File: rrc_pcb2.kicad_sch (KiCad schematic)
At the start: 15 parts, among them J1 buzzer_toggle_pin, J2 battery_header, U1 BN220-GPS, U2 INA260, U3 Teensy4.1, U4 voltReg, U5 MS5611, U6 logo

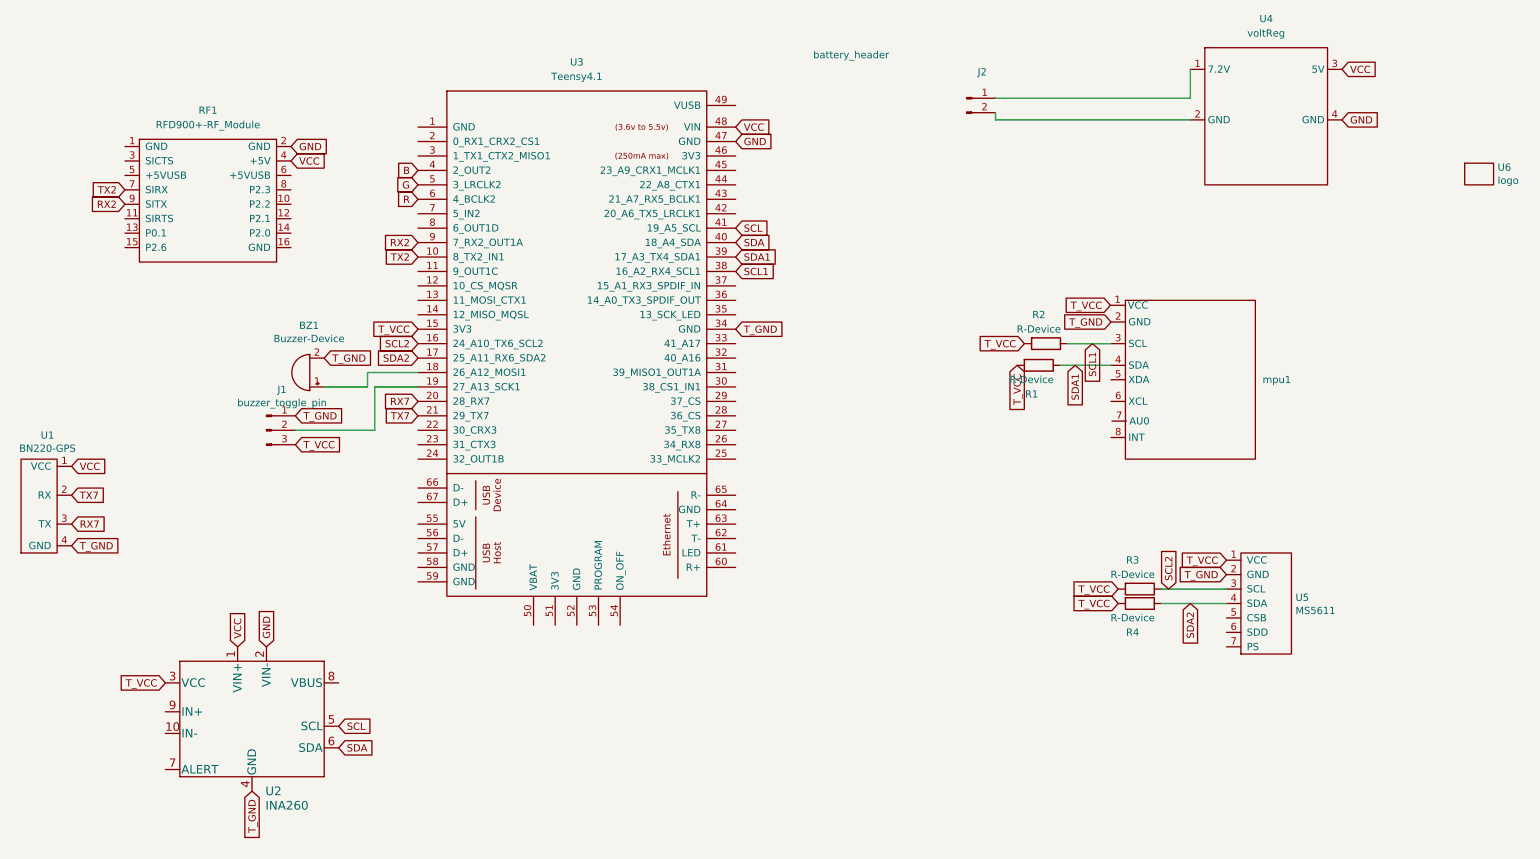
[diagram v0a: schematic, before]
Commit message: big cleanup of files
also new teensy4.1 symbo(the accurate one now) and fixed rfd900 schematic
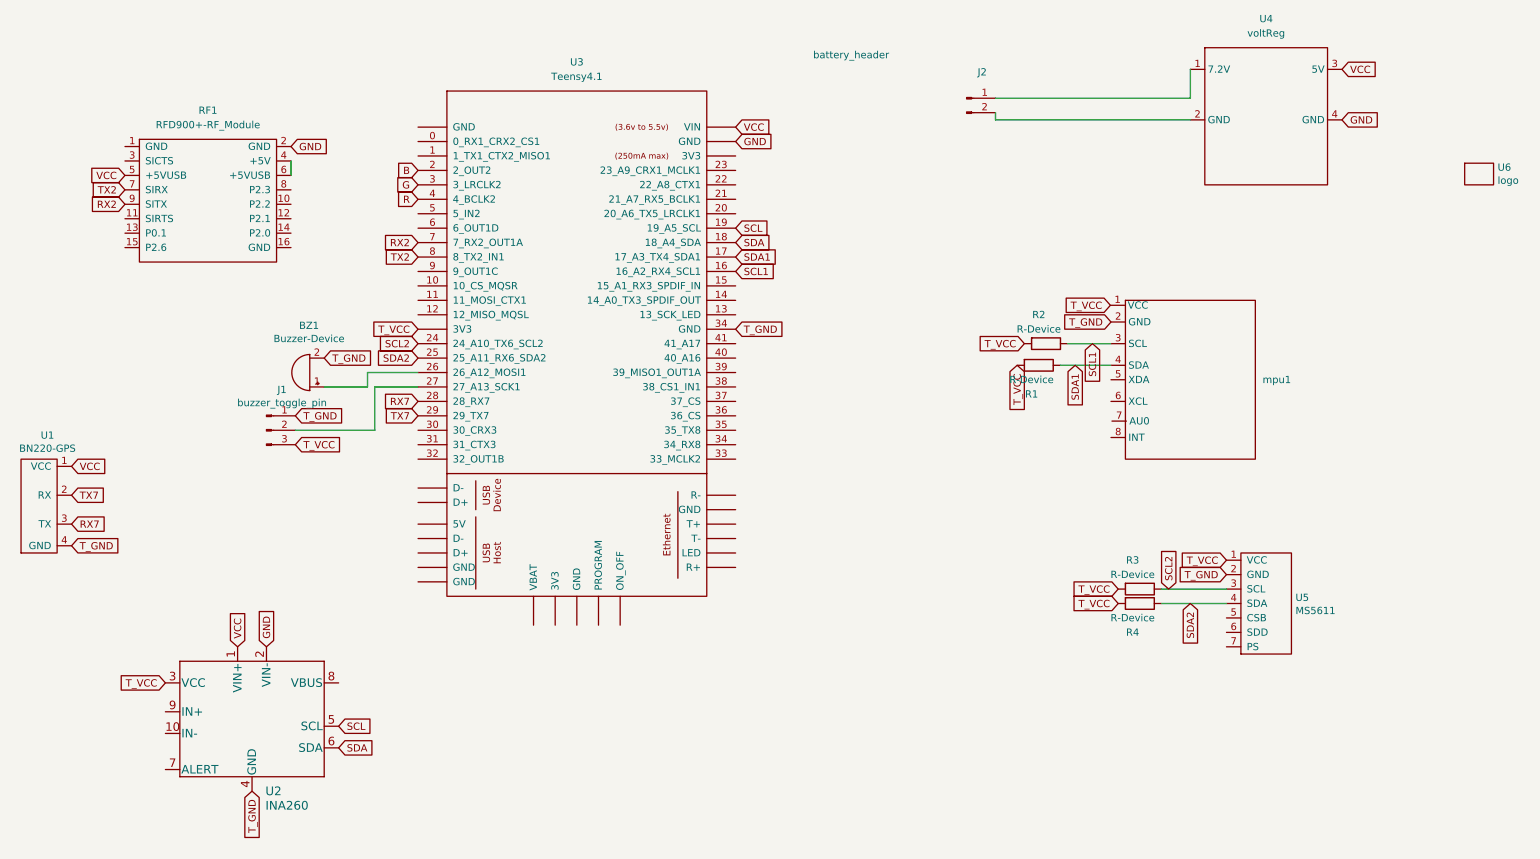
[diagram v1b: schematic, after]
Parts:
- U3: symbol teensy:Teensy4.1 -> parts:Teensy4.1
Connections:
- net B: now also U3.2 (2_OUT2); no longer U3.4 (2_OUT2)
- net G: now also U3.3 (3_LRCLK2); no longer U3.5 (3_LRCLK2)
- net GND: now also U3. (GND); no longer U3.47 (GND)
- net R: now also U3.4 (4_BCLK2); no longer U3.6 (4_BCLK2)
- net RX2: now also U3.7 (7_RX2_OUT1A); no longer U3.9 (7_RX2_OUT1A)
- net RX7: now also U3.28 (28_RX7); no longer U3.20 (28_RX7)
- net SCL: now also U3.19 (19_A5_SCL); no longer U3.41 (19_A5_SCL)
- net SCL1: now also U3.16 (16_A2_RX4_SCL1); no longer U3.38 (16_A2_RX4_SCL1)
- net SCL2: now also U3.24 (24_A10_TX6_SCL2); no longer U3.16 (24_A10_TX6_SCL2)
- net SDA: now also U3.18 (18_A4_SDA); no longer U3.40 (18_A4_SDA)
- net SDA1: now also U3.17 (17_A3_TX4_SDA1); no longer U3.39 (17_A3_TX4_SDA1)
- net SDA2: now also U3.25 (25_A11_RX6_SDA2); no longer U3.17 (25_A11_RX6_SDA2)
- net TX2: now also U3.8 (8_TX2_IN1); no longer U3.10 (8_TX2_IN1)
- net TX7: now also U3.29 (29_TX7); no longer U3.21 (29_TX7)
- net T_VCC: now also U3. (GND); no longer U3.15 (3V3)
- net VCC: now also RF1.5 (+5VUSB), U3. (GND); no longer RF1.4 (+5V), U3.48 (VIN)
- net at BZ1.1 (-): now also U3.26 (26_A12_MOSI1); no longer U3.18 (26_A12_MOSI1)
- net at J1.2 (Pin_2): now also U3.27 (27_A13_SCK1); no longer U3.19 (27_A13_SCK1)
- net at RF1.6 (+5VUSB): now also RF1.4 (+5V)
